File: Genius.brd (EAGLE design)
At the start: 218.8 x 78.7 mm, 13 parts, among them U5 ARDUINO-UNO-R3-SHIELD

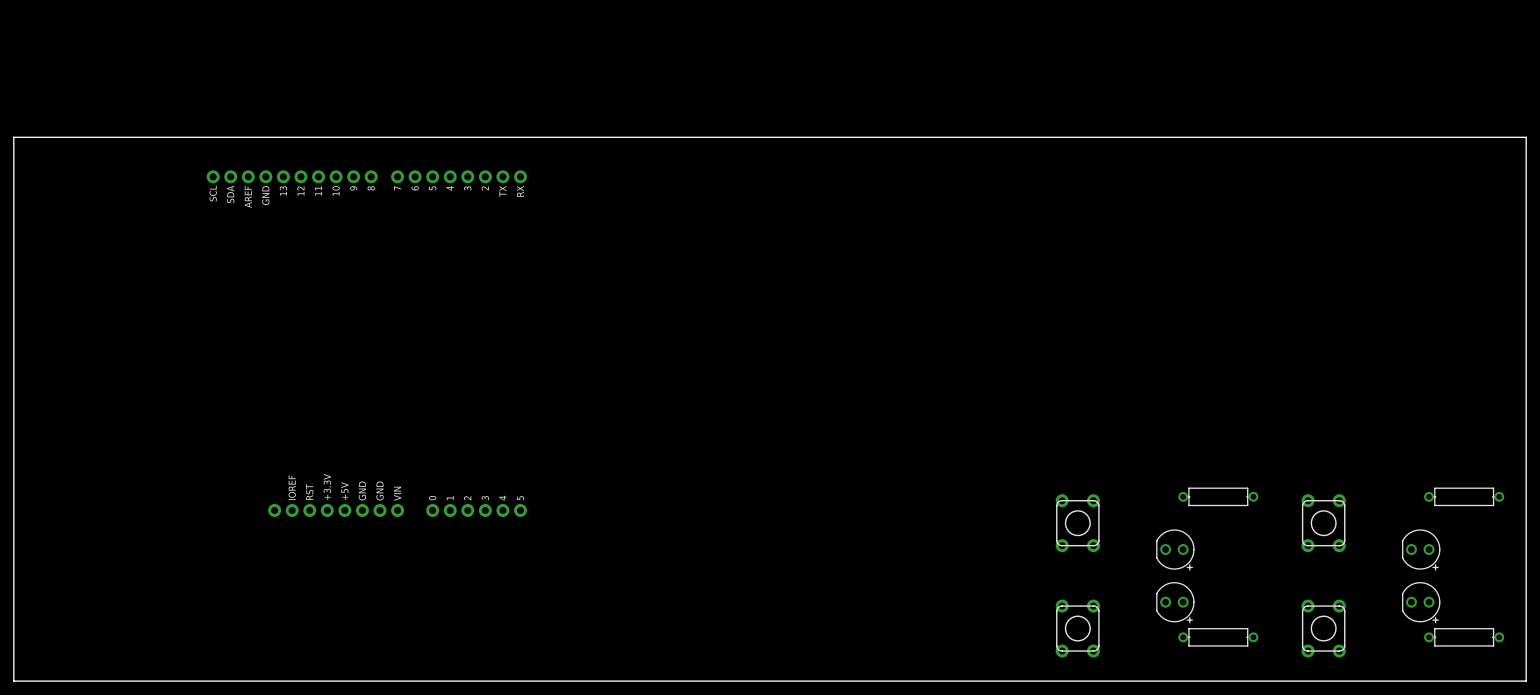
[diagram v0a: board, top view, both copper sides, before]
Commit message: 115 linhas prof ;)
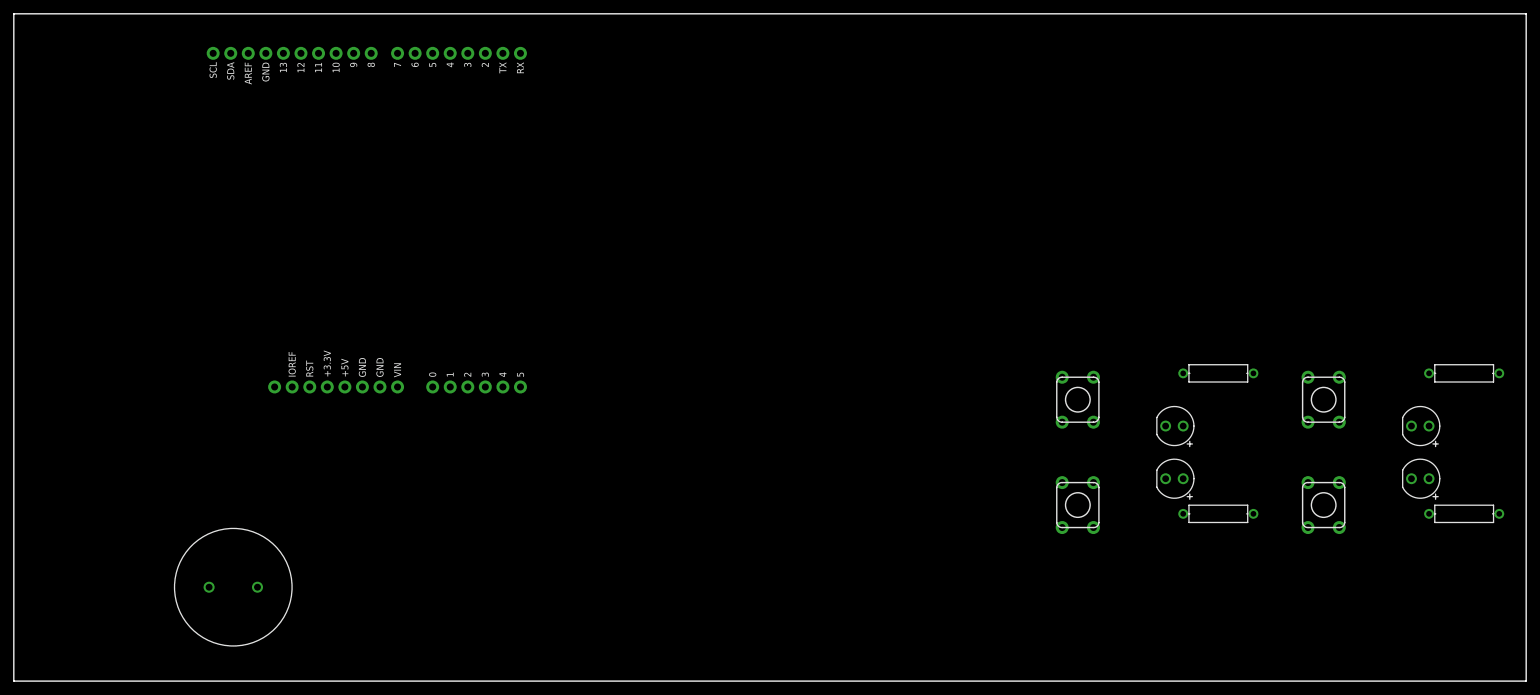
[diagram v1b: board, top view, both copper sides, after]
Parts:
- added PIEZO2: PIEZO, Tinkercad:PIEZO
- moved R1 17.9 mm to (174.2, 44.5)
- moved R2 17.9 mm to (209.8, 44.5)
- moved R3 17.9 mm to (174.2, 24.2)
- moved R4 17.9 mm to (209.8, 24.2)
- moved S2 17.9 mm to (189.5, 25.5)
- moved S3 17.9 mm to (153.9, 25.5)
- moved D1 17.9 mm to (167.9, 29.3)
- moved D2 17.9 mm to (203.4, 29.3)
- moved S1 17.9 mm to (189.5, 40.7)
- moved S4 17.9 mm to (153.9, 40.7)
- moved D3 17.9 mm to (203.4, 36.9)
- moved D4 17.9 mm to (167.9, 36.9)
- moved U5 17.9 mm to (47.9, 66.7)
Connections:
- new net U5_D10: PIEZO2.1, U5.D10
- net U5_GND: now also PIEZO2.2
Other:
- board size 218.8 x 78.7 mm -> 218.8 x 96.5 mm
